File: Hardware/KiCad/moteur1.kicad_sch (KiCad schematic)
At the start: 6 parts, among them M2 ZXBM5210-SP

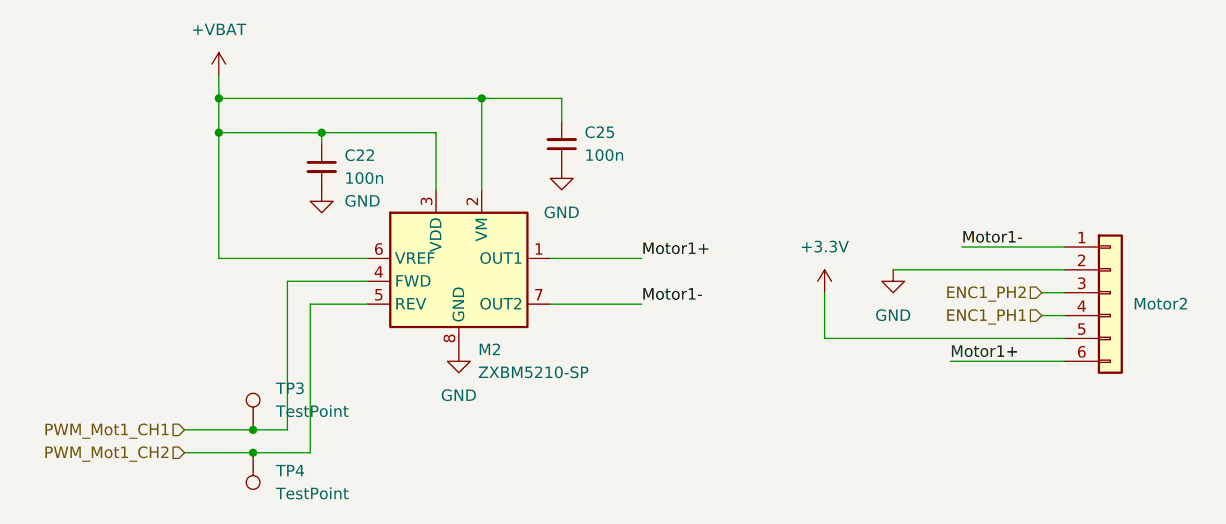
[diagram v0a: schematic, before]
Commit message: gerbers
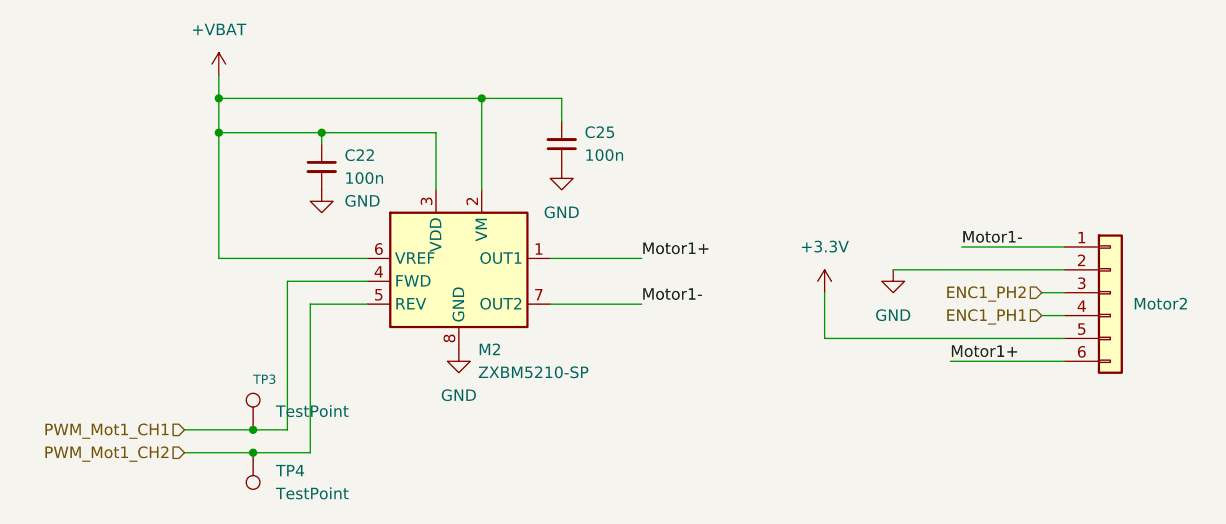
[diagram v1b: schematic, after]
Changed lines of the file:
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@@
 		(on_board yes)
 		(dnp no)
-		(fields_autoplaced yes)
 		(property "Reference" "TP3"
-			(at 106.68 93.2179 0)
+			(at 104.14 92.202 0)
 			(effects
 				(font
-					(size 1.27 1.27)
+					(size 1.016 1.016)
 				)
 				(justify left)
